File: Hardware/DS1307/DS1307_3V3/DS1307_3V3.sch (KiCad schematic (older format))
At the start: 9 parts, among them P1 I2C, U1 DS1307, X1 32.768kHz

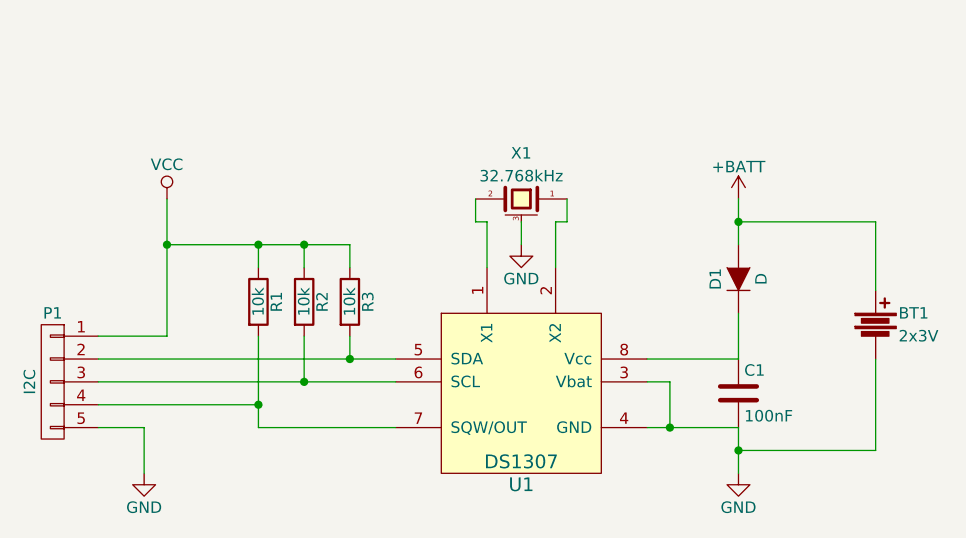
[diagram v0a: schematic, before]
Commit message: work on layout
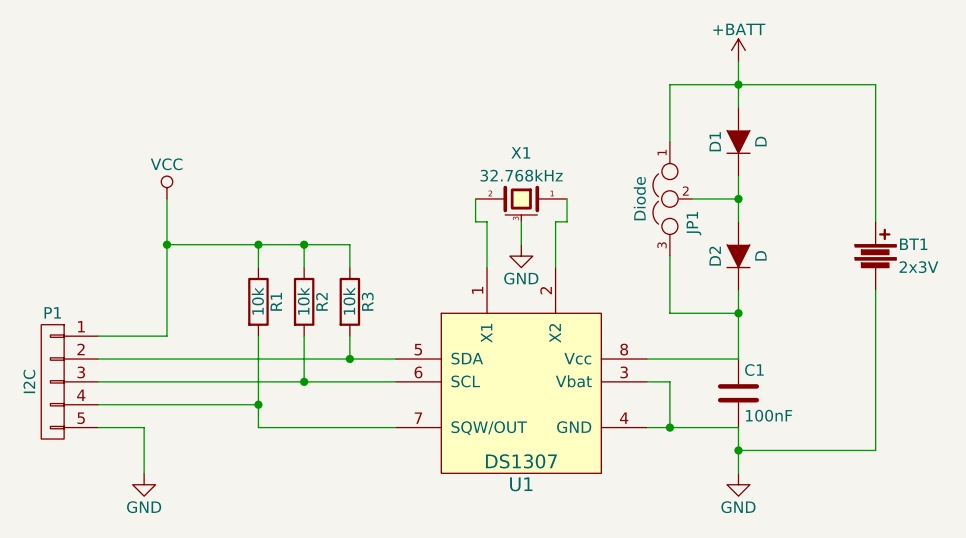
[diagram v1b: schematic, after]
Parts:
- added D2: D, Diodes_ThroughHole:Diode_DO-35_SOD27_Horizontal_RM7.5, symbol D
- added JP1: Diode, Pin_Headers:Pin_Header_Straight_1x03, symbol JUMPER3
- D1: footprint Diodes_ThroughHole:Diode_DO-35_SOD27_Horizontal_RM10 -> Diodes_ThroughHole:Diode_DO-35_SOD27_Horizontal_RM7.5
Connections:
- net +BATT: now also JP1.1
- net at C1.1, U1.8 (Vcc): now also D2.1 (K), JP1.3; no longer D1.1 (K)
- new net: D1.1 (K), D2.2 (A), JP1.2
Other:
- moved on the sheet: BT1, D1
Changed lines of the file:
@@
 LIBS:contrib
 LIBS:valves
-LIBS:ds1307
-LIBS:lp3985
 LIBS:DS1307_3V3-cache
 EELAYER 25 0
@@
 $EndComp
 Wire Wire Line
-	5700 3100 6100 3100
+	6100 3100 5700 3100
 Wire Wire Line
 	6100 3400 6100 3600
@@
 L +BATT #PWR02
 U 1 1 573CA59E
-P 6100 2400
-F 0 "#PWR02" H 6100 2250 50  0001 C CNN
-F 1 "+BATT" H 6100 2540 50  0000 C CNN
-F 2 "" H 6100 2400 60  0000 C CNN
-F 3 "" H 6100 2400 60  0000 C CNN
-	1    6100 2400
+P 6100 1800
+F 0 "#PWR02" H 6100 1650 50  0001 C CNN
+F 1 "+BATT" H 6100 1940 50  0000 C CNN
+F 2 "" H 6100 1800 60  0000 C CNN
+F 3 "" H 6100 1800 60  0000 C CNN
+	1    6100 1800
 	1    0    0    -1
 $EndComp
@@
 L D D1
 U 1 1 573CA5BE
-P 6100 2750
-F 0 "D1" H 6100 2850 50  0000 C CNN
-F 1 "D" H 6100 2650 50  0000 C CNN
-F 2 "Diodes_ThroughHole:Diode_DO-35_SOD27_Horizontal_RM10" H 6100 2750 60  0001 C CNN
-F 3 "" H 6100 2750 60  0000 C CNN
-	1    6100 2750
+P 6100 2150
+F 0 "D1" H 6100 2250 50  0000 C CNN
+F 1 "D" H 6100 2050 50  0000 C CNN
+F 2 "Diodes_ThroughHole:Diode_DO-35_SOD27_Horizontal_RM7.5" H 6100 2150 60  0001 C CNN
+F 3 "" H 6100 2150 60  0000 C CNN
+	1    6100 2150
 	0    -1   -1   0
 $EndComp
 Wire Wire Line
-	6100 2400 6100 2600
-Wire Wire Line
-	6100 3100 6100 2900
+	6100 2800 6100 3100
 $Comp
 L CONN_01X05 P1
@@
 $EndComp
 Wire Wire Line
-	6100 2500 6700 2500
-Wire Wire Line
-	6700 2500 6700 2800
-Connection ~ 6100 2500
+	5800 1900 6700 1900
+Connection ~ 6100 1900
 Wire Wire Line
 	6700 3500 6100 3500
-Wire Wire Line
-	6700 3100 6700 3500
 Connection ~ 6100 3500
 $Comp
@@
 L Battery BT1
 U 1 1 573CB2A4
-P 6700 2950
-F 0 "BT1" H 6800 3000 50  0000 L CNN
-F 1 "2x3V" H 6800 2900 50  0000 L CNN
-F 2 "KZH-20:KZH-20" V 6700 2990 60  0001 C CNN
-F 3 "" V 6700 2990 60  0000 C CNN
-	1    6700 2950
-	1    0    0    -1
-$EndComp
+P 6700 2650
+F 0 "BT1" H 6800 2700 50  0000 L CNN
+F 1 "2x3V" H 6800 2600 50  0000 L CNN
+F 2 "KZH-20:KZH-20" V 6700 2690 60  0001 C CNN
+F 3 "" V 6700 2690 60  0000 C CNN
+	1    6700 2650
+	1    0    0    -1
+$EndComp
+$Comp
+L D D2
+U 1 1 574F2753
+P 6100 2650
+F 0 "D2" H 6100 2750 50  0000 C CNN
+F 1 "D" H 6100 2550 50  0000 C CNN
+F 2 "Diodes_ThroughHole:Diode_DO-35_SOD27_Horizontal_RM7.5" H 6100 2650 60  0001 C CNN
+F 3 "" H 6100 2650 60  0000 C CNN
+	1    6100 2650
+	0    -1   -1   0
+$EndComp
+$Comp
+L JUMPER3 JP1
+U 1 1 57526D20
+P 5800 2400
+F 0 "JP1" H 5850 2300 50  0000 L CNN
+F 1 "Diode" H 5800 2500 50  0000 C BNN
+F 2 "Pin_Headers:Pin_Header_Straight_1x03" H 5800 2400 50  0001 C CNN
+F 3 "" H 5800 2400 50  0000 C CNN
+	1    5800 2400
+	0    -1   1    0
+$EndComp
+Wire Wire Line
+	5900 2400 6100 2400
+Wire Wire Line
+	6100 2300 6100 2500
+Connection ~ 6100 2400
+Wire Wire Line
+	6100 2000 6100 1800
+Wire Wire Line
+	6700 1900 6700 2500
+Wire Wire Line
+	6700 2800 6700 3500
+Wire Wire Line
+	6100 2900 5800 2900
+Connection ~ 6100 2900
+Wire Wire Line
+	5800 2900 5800 2650
+Wire Wire Line
+	5800 2150 5800 1900
 $EndSCHEMATC
